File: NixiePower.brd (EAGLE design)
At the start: 66 x 38.7 mm, 21 parts, among them IC1 MC34063AD, T1 MJD31

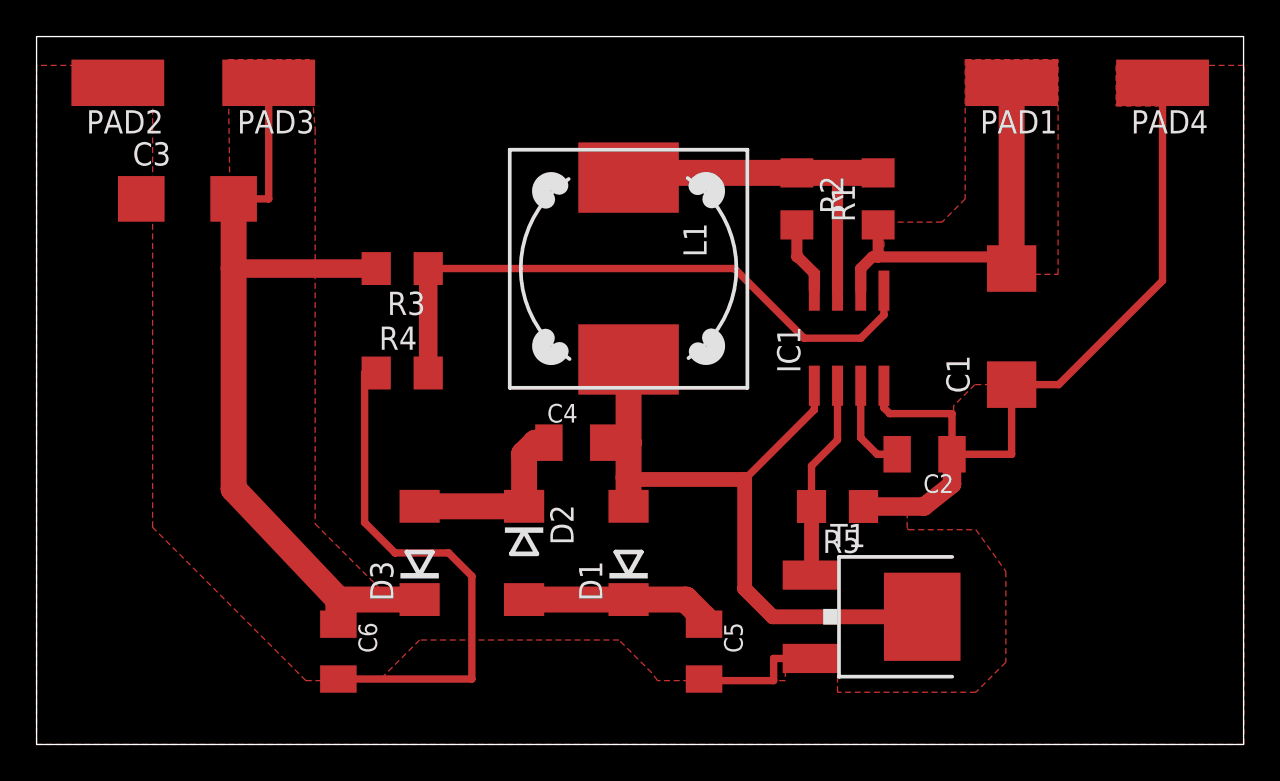
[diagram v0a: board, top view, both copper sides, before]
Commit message: Commit of Rev.C version
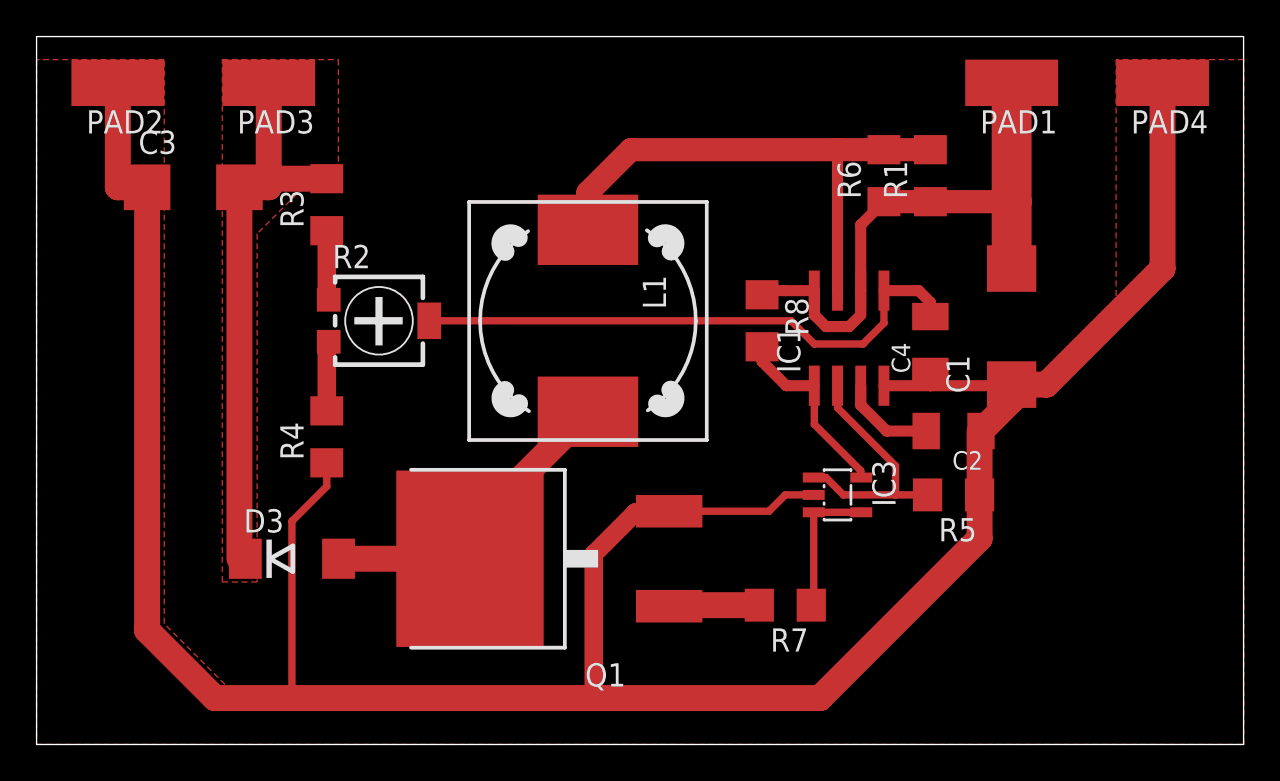
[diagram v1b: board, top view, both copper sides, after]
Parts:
- removed C5, C6: 470nF, rcl:C1206K
- removed D1, D2: MURS120, diode:DO214AA
- removed T1: MJD31, transistor:DPAK
- added IC3: IRS44273L, own-collection:SOT23-5
- added Q1: IRF740D2PAK, own-collection:D2PAK
- added R6: 0.75, rcl-2:R1206
- added R7: 20, rcl-2:R1206
- added R8: 0, rcl-2:R1206
- C2: value 400pF -> 470pF
- C4: value 470nF -> 0.1uF
- L1: value DR125 -> 220uH
- R1: value 0.5 -> 0.75
- R2: value 180 -> 20k; device rcl-2:R1206 -> rcl:RTRIM4G/J
- R3: value 47k -> 560k
- R4: value 2.2k -> 3.3k
- R5: value (none) -> 1.5k
- moved R2 23.8 mm to (18.7, 23.2)
- moved C4 20.1 mm to (48.9, 21.9), turned to 90 degrees
- moved D3 6.99 mm to (14.0, 10.2), turned to 0 degrees
- moved R5 6.38 mm to (50.2, 13.7)
- moved R3 5.41 mm to (15.9, 29.5), turned to 90 degrees
- moved R4 5.41 mm to (15.9, 16.8), turned to 90 degrees
- moved L1 3.62 mm to (30.2, 23.2)
- moved R1 3.13 mm to (48.9, 31.1)
- moved C2 2.03 mm to (50.2, 17.1)
- moved C3 0.71 mm to (8.57, 30.5)
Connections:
- new net N$6: C3.+, D3.C, PAD3.1, R3.2
- new net VCC: C1.+, IC1.6, IC1.8, PAD1.1, R1.1, R6.1, R8.1
- net GND: now also C4.1, IC3.2, Q1.3; no longer C5.2, C6.2, T1.3
- net N$1: now also D3.A, Q1.4; no longer C4.2, D1.A, IC1.1, T1.4
- net N$10: now also R2.3, R4.2; no longer C3.+, C6.1, D3.C, PAD3.1, R3.2
- net N$11: now also IC3.1; no longer T1.1
- net N$3: now also R6.2; no longer R2.1
- net N$4: now also IC1.1, IC3.5, R8.2; no longer IC1.8, R2.2
- net N$5: now also Q1.1, R7.2; no longer C1.+, IC1.6, PAD1.1, R1.1
- net N$7: now also C4.2, R2.2; no longer R3.1, R4.2
- net N$8: now also IC3.3, IC3.4, R7.1; no longer C5.1, D1.C, D2.A
- net N$9: now also R2.1, R3.1; no longer C4.1, D2.C, D3.A
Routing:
- net GND: track 78.7 -> 156.5 mm
- net N$10: track 46.1 -> 3.89 mm
- net VCC: track 0.00 -> 31.4 mm
- net N$6: track 0.00 -> 31.3 mm
- net N$1: track 38.9 -> 17.9 mm
- net N$5: track 21.6 -> 4.93 mm
- net N$3: track 20.4 -> 29.5 mm
- net N$9: track 10.2 -> 3.89 mm
- net N$4: track 4.02 -> 10.3 mm
- net N$11: track 11.0 -> 13.9 mm
- net N$7: track 34.1 -> 31.2 mm
- net N$8: track 10.6 -> 8.35 mm
- added copper zone on layer 1, net N$6
- removed copper zone on layer 1, net N$10
- removed copper zone on layer 1, net N$5
